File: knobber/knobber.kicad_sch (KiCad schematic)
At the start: 1 part, among them J102 BLDC

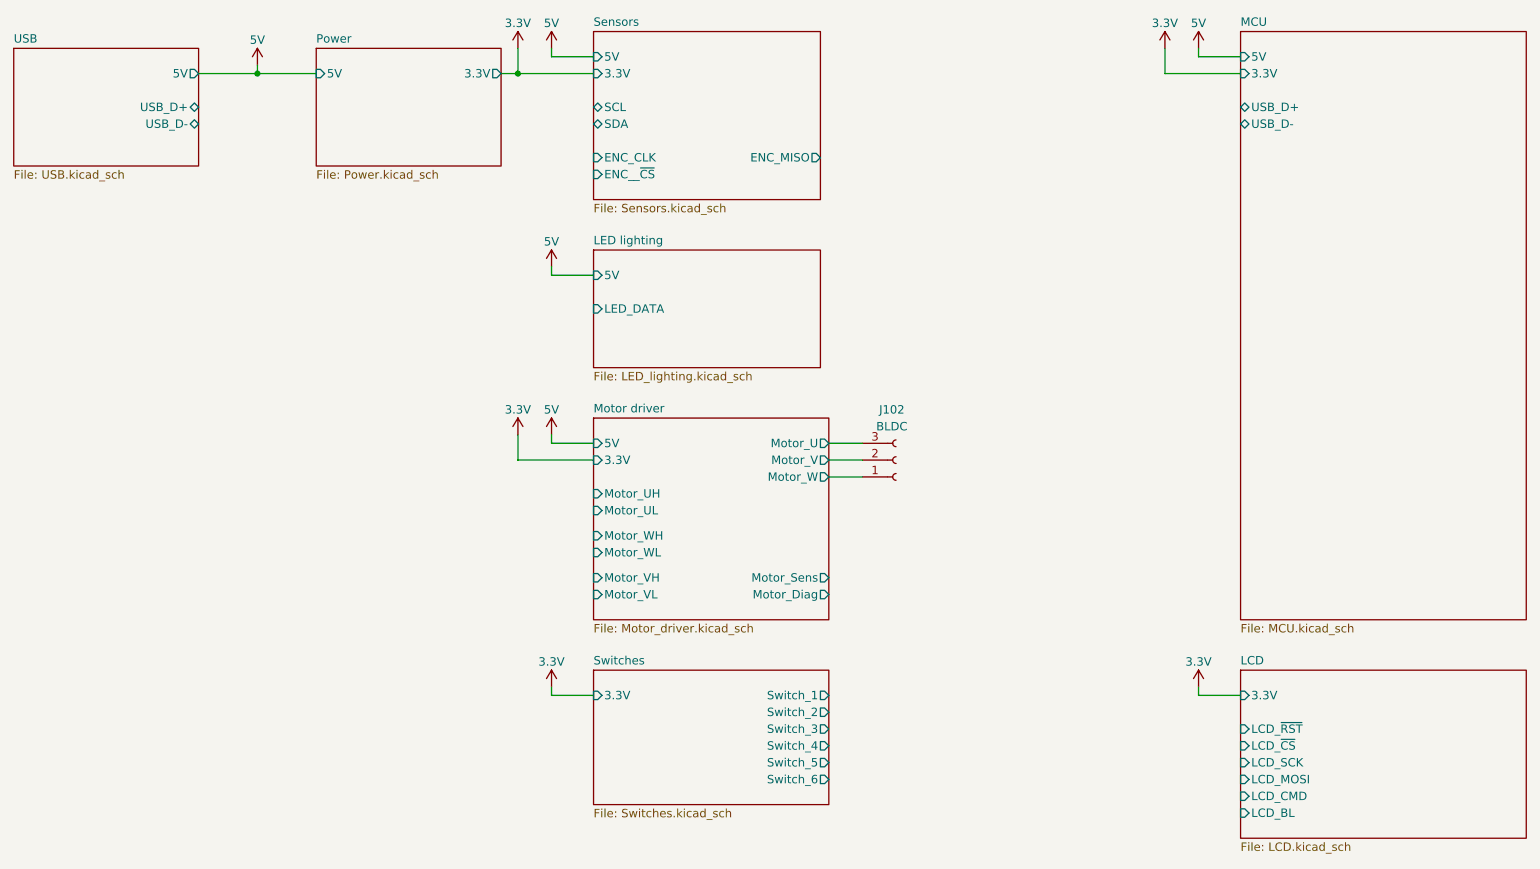
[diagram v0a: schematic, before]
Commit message: updated schematic
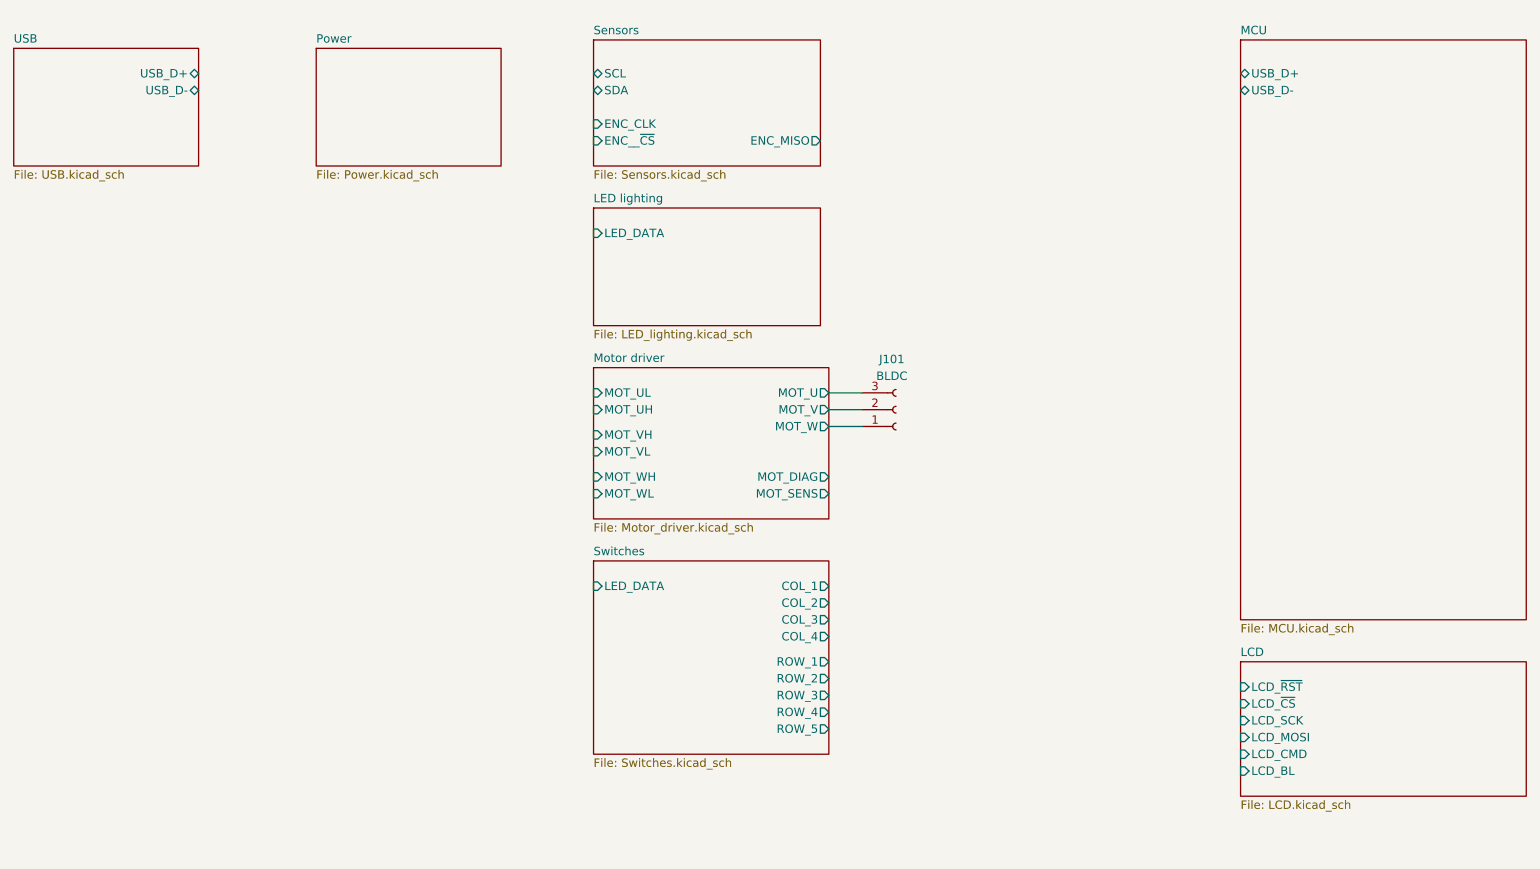
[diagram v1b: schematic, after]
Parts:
- J101: renamed from J102; footprint (none) -> Connector_Molex:Molex_SPOX_5267-03A_1x03_P2.50mm_Vertical
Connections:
- net Motor driver/Motor_U renamed Motor driver/MOT_U
- net Motor driver/Motor_V renamed Motor driver/MOT_V
- net Motor driver/Motor_W renamed Motor driver/MOT_W
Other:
- sheet LCD ports: added none; removed 3.3V
- sheet LED lighting ports: added none; removed 5V
- sheet MCU ports: added none; removed 3.3V, 5V
- sheet Motor driver ports: added MOT_DIAG, MOT_SENS, MOT_U, MOT_UH, MOT_UL, MOT_V, MOT_VH, MOT_VL, MOT_W, MOT_WH, MOT_WL; removed 3.3V, 5V, Motor_Diag, Motor_Sens, Motor_U, Motor_UH, Motor_UL, Motor_V, Motor_VH, Motor_VL, Motor_W, Motor_WH, Motor_WL
- sheet Power ports: added none; removed 3.3V, 5V
- sheet Sensors ports: added none; removed 3.3V, 5V
- sheet Switches ports: added COL_1, COL_2, COL_3, COL_4, LED_DATA, ROW_1, ROW_2, ROW_3, ROW_4, ROW_5; removed 3.3V, Switch_1, Switch_2, Switch_3, Switch_4, Switch_5, Switch_6
- sheet USB ports: added none; removed 5V
- moved on the sheet: J101
